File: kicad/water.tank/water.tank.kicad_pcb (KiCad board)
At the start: 2 copper layers, 7 parts, among them J1 ESP8266, J5 5V, U1 LD33V

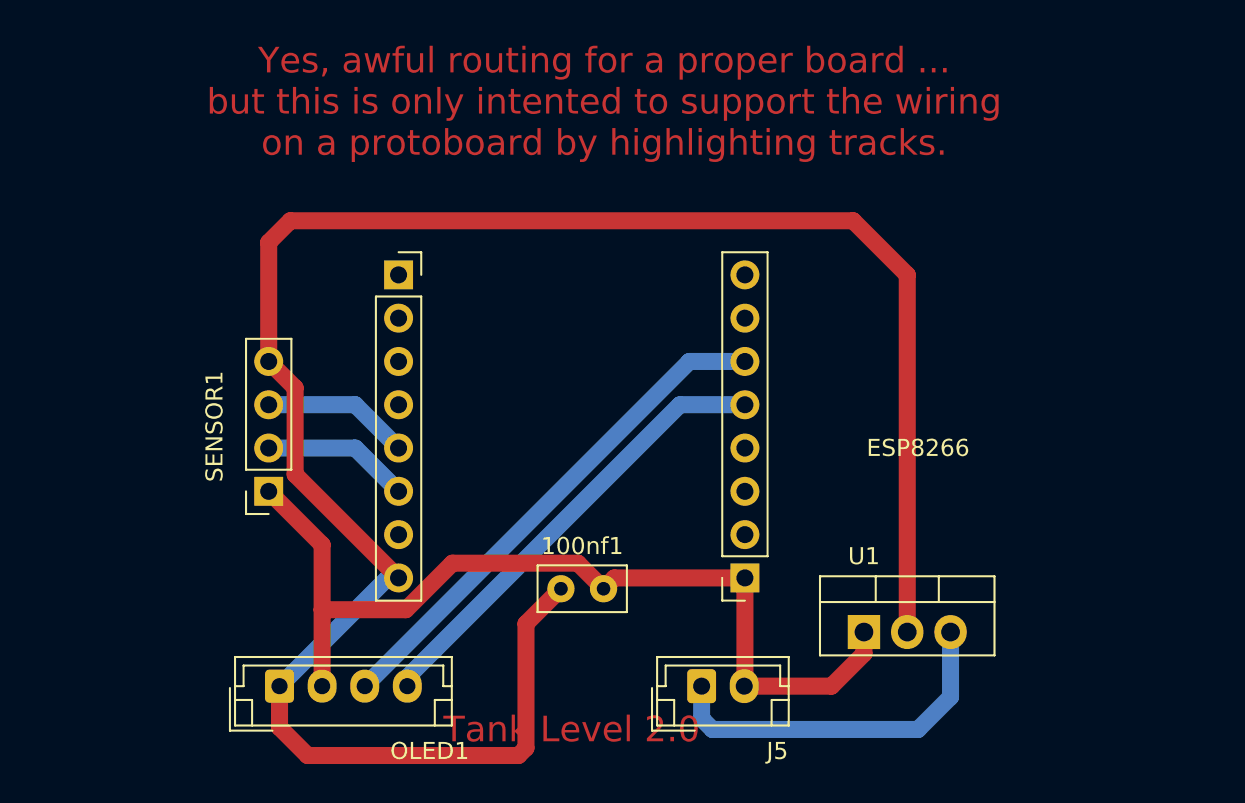
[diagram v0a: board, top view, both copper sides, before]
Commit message: a few unrelated things
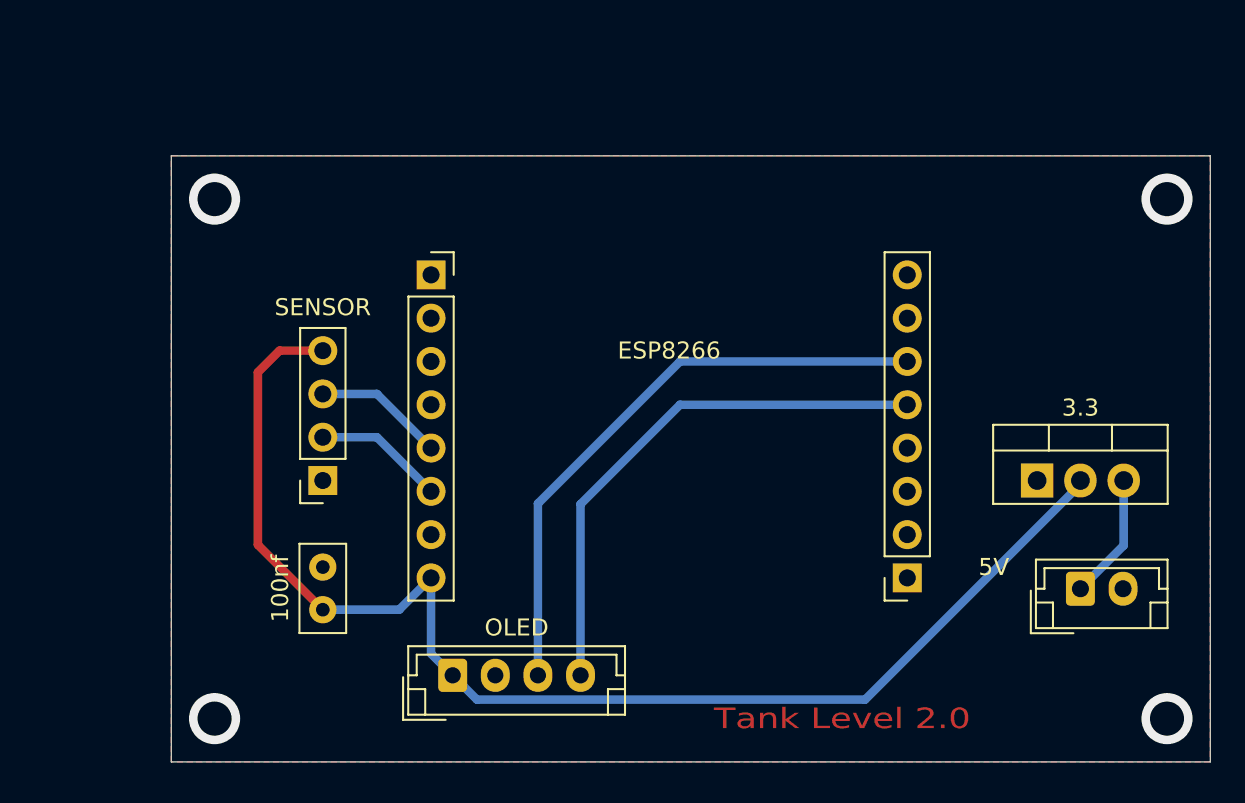
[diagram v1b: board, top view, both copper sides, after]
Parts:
- removed 100nf1: CAP, Capacitor_THT:C_Disc_D5.0mm_W2.5mm_P2.50mm
- removed J5: 5V, Connector_JST:JST_EH_B2B-EH-A_1x02_P2.50mm_Vertical
- removed OLED1: OLED, Connector_JST:JST_EH_B4B-EH-A_1x04_P2.50mm_Vertical
- removed SENSOR1: SENSOR, Connector_PinSocket_2.54mm:PinSocket_1x04_P2.54mm_Vertical
- removed U1: LD33V, Package_TO_SOT_THT:TO-220-3_Vertical
- added 100nf: CAP, Capacitor_THT:C_Disc_D5.0mm_W2.5mm_P2.50mm, F.Cu at (72.4, 74.9)
- added 3.3: LD33V, Package_TO_SOT_THT:TO-220-3_Vertical, F.Cu at (114.3, 67.3)
- added 5V: source, Connector_JST:JST_EH_B2B-EH-A_1x02_P2.50mm_Vertical, F.Cu at (116.8, 73.7)
- added OLED: OLED1, Connector_JST:JST_EH_B4B-EH-A_1x04_P2.50mm_Vertical, F.Cu at (80.0, 78.7)
- added SENSOR: r, Connector_PinSocket_2.54mm:PinSocket_1x04_P2.54mm_Vertical, F.Cu at (72.4, 67.3)
- moved ESP8266 9.53 mm to (106.7, 73.0)
- moved J1 1.91 mm to (78.7, 55.2)
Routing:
- net GND: track 55.6 -> 0.00 mm
- net VCC: track 120.7 -> 76.1 mm
- net 5V: track 21.4 -> 7.40 mm
- net IO05: track 30.2 -> 35.2 mm
- net IO04: track 26.9 -> 31.6 mm
- net IO14: track 8.67 -> 7.67 mm
- net IO12: track 8.67 -> 7.67 mm
- net (no net): vias 0 -> 4
- added copper zone on F.Cu, net GND
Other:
- board outline added: 61 x 35.6 mm
- board text removed: "Yes, awful routing for a proper board ... but this is only intented to support the wiring on a protoboard by highlighting tracks."
